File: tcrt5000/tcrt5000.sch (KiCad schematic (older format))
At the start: 7 parts, among them Q1 BC817, U1 TCRT5000, X1 Conn_01x03_Male

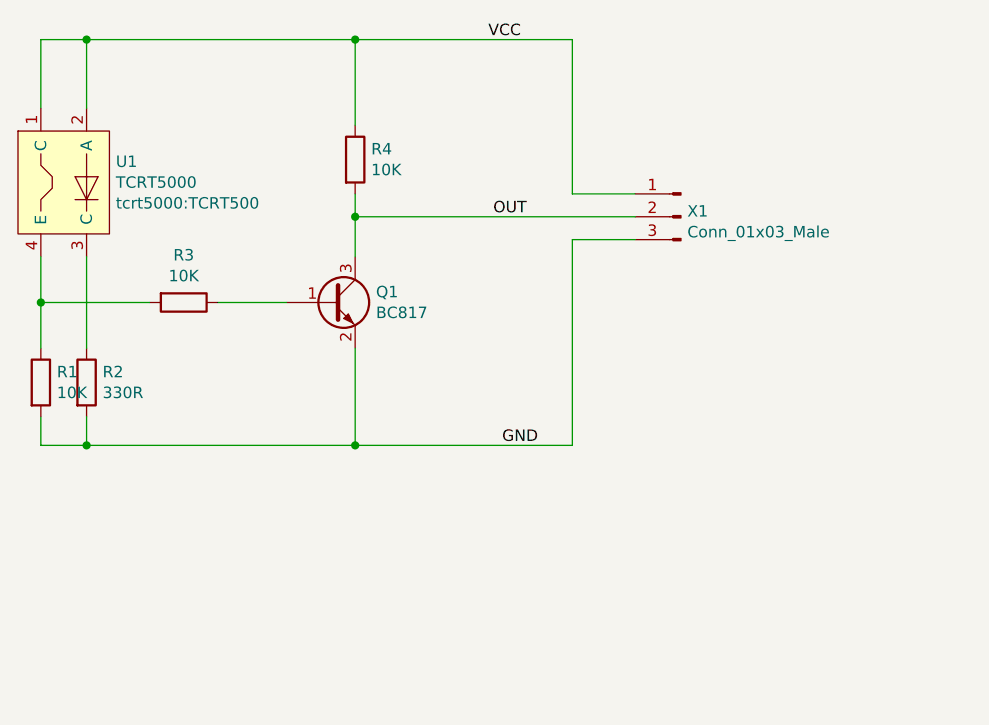
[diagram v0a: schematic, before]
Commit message: Gerbers done
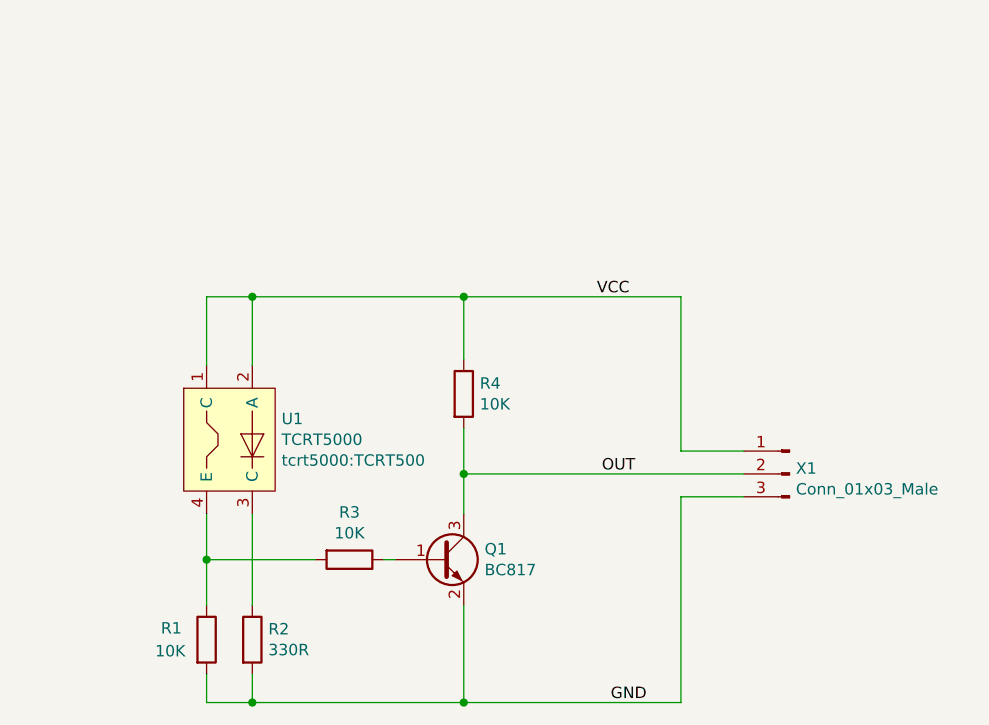
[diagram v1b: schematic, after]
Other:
- moved on the sheet: Q1, R1, R2, R3, R4, U1, X1
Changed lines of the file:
@@
 L tcrt5000:TCRT5000 U1
 U 1 1 5E29CC7F
-P 3925 2425
-F 0 "U1" H 4153 2491 50  0000 L CNN
-F 1 "TCRT5000" H 4153 2400 50  0000 L CNN
-F 2 "tcrt5000:TCRT500" H 4153 2309 50  0000 L CNN
-F 3 "" H 3925 2375 50  0001 C CNN
-	1    3925 2425
+P 4650 3550
+F 0 "U1" H 4878 3616 50  0000 L CNN
+F 1 "TCRT5000" H 4878 3525 50  0000 L CNN
+F 2 "tcrt5000:TCRT500" H 4878 3434 50  0000 L CNN
+F 3 "" H 4650 3500 50  0001 C CNN
+	1    4650 3550
 	1    0    0    -1
 $EndComp
 Wire Wire Line
-	3825 2125 3825 1825
+	4550 3250 4550 2950
 Wire Wire Line
-	3825 1825 4025 1825
+	4550 2950 4750 2950
 Wire Wire Line
-	4025 2125 4025 1825
-Connection ~ 4025 1825
+	4750 3250 4750 2950
+Connection ~ 4750 2950
 $Comp
 L Device:R R2
 U 1 1 5E29DACB
-P 4025 3325
-F 0 "R2" H 4095 3371 50  0000 L CNN
-F 1 "330R" H 4095 3280 50  0000 L CNN
-F 2 "Resistor_SMD:R_0805_2012Metric" V 3955 3325 50  0001 C CNN
-F 3 "~" H 4025 3325 50  0001 C CNN
-	1    4025 3325
+P 4750 4450
+F 0 "R2" H 4820 4496 50  0000 L CNN
+F 1 "330R" H 4820 4405 50  0000 L CNN
+F 2 "Resistor_SMD:R_0805_2012Metric" V 4680 4450 50  0001 C CNN
+F 3 "~" H 4750 4450 50  0001 C CNN
+	1    4750 4450
 	1    0    0    -1
 $EndComp
@@
 L Device:R R1
 U 1 1 5E29DF88
-P 3825 3325
-F 0 "R1" H 3895 3371 50  0000 L CNN
-F 1 "10K" H 3895 3280 50  0000 L CNN
-F 2 "Resistor_SMD:R_0805_2012Metric" V 3755 3325 50  0001 C CNN
-F 3 "~" H 3825 3325 50  0001 C CNN
-	1    3825 3325
+P 4550 4450
+F 0 "R1" H 4350 4500 50  0000 L CNN
+F 1 "10K" H 4325 4400 50  0000 L CNN
+F 2 "Resistor_SMD:R_0805_2012Metric" V 4480 4450 50  0001 C CNN
+F 3 "~" H 4550 4450 50  0001 C CNN
+	1    4550 4450
 	1    0    0    -1
 $EndComp
 Wire Wire Line
-	3825 3475 3825 3600
+	4550 4600 4550 4725
 Wire Wire Line
-	3825 3600 4025 3600
+	4550 4725 4750 4725
 Wire Wire Line
-	4025 3475 4025 3600
-Connection ~ 4025 3600
+	4750 4600 4750 4725
+Connection ~ 4750 4725
 Wire Wire Line
-	3825 3175 3825 2975
+	4550 4300 4550 4100
 Wire Wire Line
-	4025 2775 4025 3175
+	4750 3900 4750 4300
 Wire Wire Line
-	3825 2975 4300 2975
-Connection ~ 3825 2975
+	4550 4100 5025 4100
+Connection ~ 4550 4100
 Wire Wire Line
-	3825 2975 3825 2775
+	4550 4100 4550 3900
 $Comp
 L Device:R R3
 U 1 1 5E29E5DC
-P 4450 2975
-F 0 "R3" V 4243 2975 50  0000 C CNN
-F 1 "10K" V 4334 2975 50  0000 C CNN
-F 2 "Resistor_SMD:R_0805_2012Metric" V 4380 2975 50  0001 C CNN
-F 3 "~" H 4450 2975 50  0001 C CNN
-	1    4450 2975
+P 5175 4100
+F 0 "R3" V 4968 4100 50  0000 C CNN
+F 1 "10K" V 5059 4100 50  0000 C CNN
+F 2 "Resistor_SMD:R_0805_2012Metric" V 5105 4100 50  0001 C CNN
+F 3 "~" H 5175 4100 50  0001 C CNN
+	1    5175 4100
 	0    1    1    0
 $EndComp
 Wire Wire Line
-	4600 2975 4900 2975
+	5325 4100 5375 4100
 $Comp
 L Transistor_BJT:BC817 Q1
 U 1 1 5E29F24F
-P 5100 2975
-F 0 "Q1" H 5291 3021 50  0000 L CNN
-F 1 "BC817" H 5291 2930 50  0000 L CNN
-F 2 "Package_TO_SOT_SMD:SOT-23" H 5300 2900 50  0001 L CIN
-F 3 "http://www.fairchildsemi.com/ds/BC/BC817.pdf" H 5100 2975 50  0001 L CNN
-	1    5100 2975
+P 5575 4100
+F 0 "Q1" H 5766 4146 50  0000 L CNN
+F 1 "BC817" H 5766 4055 50  0000 L CNN
+F 2 "Package_TO_SOT_SMD:SOT-23" H 5775 4025 50  0001 L CIN
+F 3 "http://www.fairchildsemi.com/ds/BC/BC817.pdf" H 5575 4100 50  0001 L CNN
+	1    5575 4100
 	1    0    0    -1
 $EndComp
 Wire Wire Line
-	5200 3175 5200 3600
+	5675 4300 5675 4725
 Wire Wire Line
-	4025 3600 5200 3600
+	4750 4725 5675 4725
 $Comp
 L Device:R R4
 U 1 1 5E29FB00
-P 5200 2350
-F 0 "R4" H 5270 2396 50  0000 L CNN
-F 1 "10K" H 5270 2305 50  0000 L CNN
-F 2 "Resistor_SMD:R_0805_2012Metric" V 5130 2350 50  0001 C CNN
-F 3 "~" H 5200 2350 50  0001 C CNN
-	1    5200 2350
+P 5675 3375
+F 0 "R4" H 5745 3421 50  0000 L CNN
+F 1 "10K" H 5745 3330 50  0000 L CNN
+F 2 "Resistor_SMD:R_0805_2012Metric" V 5605 3375 50  0001 C CNN
+F 3 "~" H 5675 3375 50  0001 C CNN
+	1    5675 3375
 	1    0    0    -1
 $EndComp
 Wire Wire Line
-	5200 2500 5200 2600
+	5675 3525 5675 3725
 Wire Wire Line
-	5200 2200 5200 1825
+	5675 3225 5675 2950
 Wire Wire Line
-	4025 1825 5200 1825
-Connection ~ 5200 1825
-Connection ~ 5200 2600
+	4750 2950 5675 2950
+Connection ~ 5675 2950
+Connection ~ 5675 3725
 Wire Wire Line
-	5200 2600 5200 2775
-Connection ~ 5200 3600
+	5675 3725 5675 3900
+Connection ~ 5675 4725
 $Comp
 L Connector:Conn_01x03_Male X1
 U 1 1 5E2A6981
-P 6625 2600
-F 0 "X1" H 6597 2624 50  0000 R CNN
-F 1 "Conn_01x03_Male" H 6597 2533 50  0000 R CNN
-F 2 "Connector_PinHeader_2.54mm:PinHeader_1x03_P2.54mm_Vertical" H 6625 2600 50  0001 C CNN
-F 3 "~" H 6625 2600 50  0001 C CNN
-	1    6625 2600
+P 7100 3725
+F 0 "X1" H 7072 3749 50  0000 R CNN
+F 1 "Conn_01x03_Male" H 7072 3658 50  0000 R CNN
+F 2 "Connector_PinHeader_2.54mm:PinHeader_1x03_P2.54mm_Vertical" H 7100 3725 50  0001 C CNN
+F 3 "~" H 7100 3725 50  0001 C CNN
+	1    7100 3725
 	-1   0    0    -1
 $EndComp
-Text Label 5925 1825 2    50   ~ 0
+Text Label 6400 2950 2    50   ~ 0
 VCC
-Text Label 5950 2600 2    50   ~ 0
+Text Label 6425 3725 2    50   ~ 0
 OUT
-Text Label 6000 3600 2    50   ~ 0
+Text Label 6475 4725 2    50   ~ 0
 GND
 Wire Wire Line
-	6150 1825 6150 2500
+	6625 2950 6625 3625
 Wire Wire Line
-	6150 2500 6425 2500
+	6625 3625 6900 3625
 Wire Wire Line
-	5200 1825 6150 1825
+	5675 2950 6625 2950
 Wire Wire Line
-	5200 2600 6425 2600
+	5675 3725 6900 3725
 Wire Wire Line
-	6150 3600 6150 2700
+	6625 4725 6625 3825
 Wire Wire Line
-	6150 2700 6425 2700
+	6625 3825 6900 3825
 Wire Wire Line
-	5200 3600 6150 3600
+	5675 4725 6625 4725
 $EndSCHEMATC
